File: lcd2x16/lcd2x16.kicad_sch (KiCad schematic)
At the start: 7 parts, among them U1 74HC688, U2 74HC02

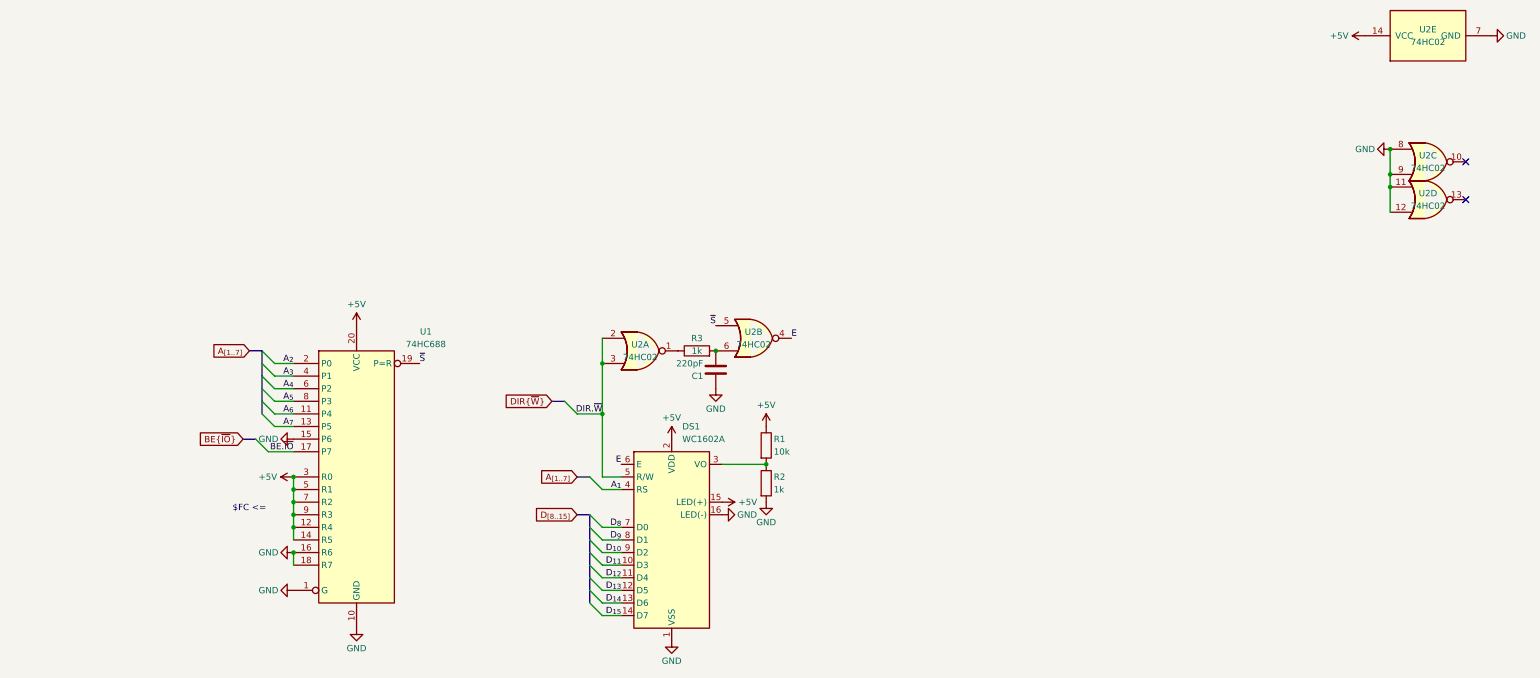
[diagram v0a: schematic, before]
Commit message: lcd2x16 ready
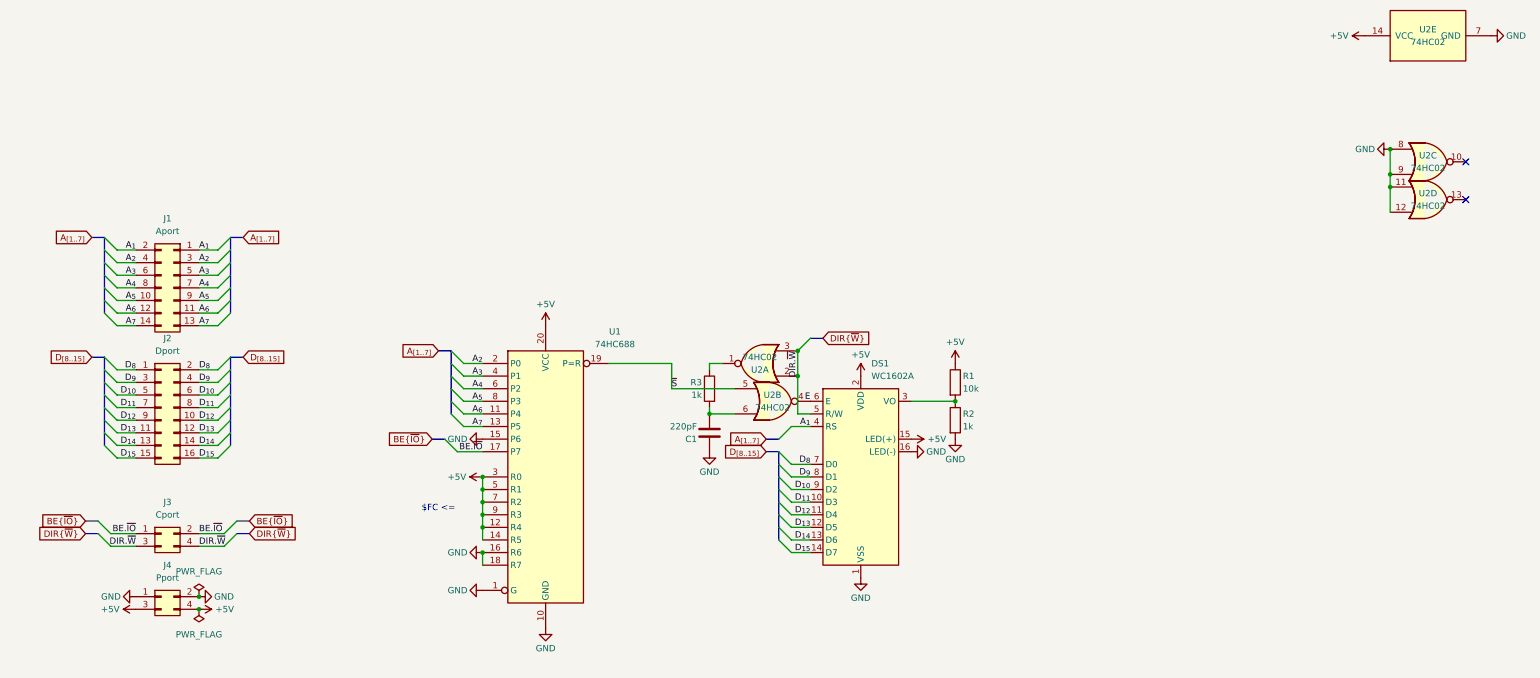
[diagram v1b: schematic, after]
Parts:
- added J1: Aport, Connector_PinSocket_2.54mm:PinSocket_2x07_P2.54mm_Vertical, symbol Connector_Generic:Conn_02x07_Odd_Even
- added J2: Dport, Connector_PinSocket_2.54mm:PinSocket_2x08_P2.54mm_Vertical, symbol Connector_Generic:Conn_02x08_Odd_Even
- added J3: Cport, Connector_PinSocket_2.54mm:PinSocket_2x02_P2.54mm_Vertical, symbol Connector_Generic:Conn_02x02_Odd_Even
- added J4: Pport, Connector_PinSocket_2.54mm:PinSocket_2x02_P2.54mm_Vertical, symbol Connector_Generic:Conn_02x02_Odd_Even
- C1: footprint (none) -> Capacitor_THT:C_Disc_D3.0mm_W1.6mm_P2.54mm
- R1, R2, R3: footprint (none) -> Resistor_THT:R_Axial_DIN0207_L6.3mm_D2.5mm_P7.62mm_Horizontal
- U1: footprint (none) -> Package_DIP:DIP-20_W7.62mm
- U2: footprint (none) -> Package_DIP:DIP-14_W7.62mm
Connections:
- net +5V: now also J4.3 (Pin_3), J4.4 (Pin_4)
- net A_{1}: now also J1.1 (Pin_1), J1.2 (Pin_2)
- net A_{2}: now also J1.3 (Pin_3), J1.4 (Pin_4)
- net A_{3}: now also J1.5 (Pin_5), J1.6 (Pin_6)
- net A_{4}: now also J1.7 (Pin_7), J1.8 (Pin_8)
- net A_{5}: now also J1.10 (Pin_10), J1.9 (Pin_9)
- net A_{6}: now also J1.11 (Pin_11), J1.12 (Pin_12)
- net A_{7}: now also J1.13 (Pin_13), J1.14 (Pin_14)
- net BE.~{IO}: now also J3.1 (Pin_1), J3.2 (Pin_2)
- net DIR.~{W}: now also J3.3 (Pin_3), J3.4 (Pin_4)
- net D_{10}: now also J2.5 (Pin_5), J2.6 (Pin_6)
- net D_{11}: now also J2.7 (Pin_7), J2.8 (Pin_8)
- net D_{12}: now also J2.10 (Pin_10), J2.9 (Pin_9)
- net D_{13}: now also J2.11 (Pin_11), J2.12 (Pin_12)
- net D_{14}: now also J2.13 (Pin_13), J2.14 (Pin_14)
- net D_{15}: now also J2.15 (Pin_15), J2.16 (Pin_16)
- net D_{8}: now also J2.1 (Pin_1), J2.2 (Pin_2)
- net D_{9}: now also J2.3 (Pin_3), J2.4 (Pin_4)
- net GND: now also J4.1 (Pin_1), J4.2 (Pin_2)
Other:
- moved on the sheet: C1, DS1, R1, R2, U1, U2A, U2B
